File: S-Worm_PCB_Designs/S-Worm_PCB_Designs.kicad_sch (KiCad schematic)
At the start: 25 parts

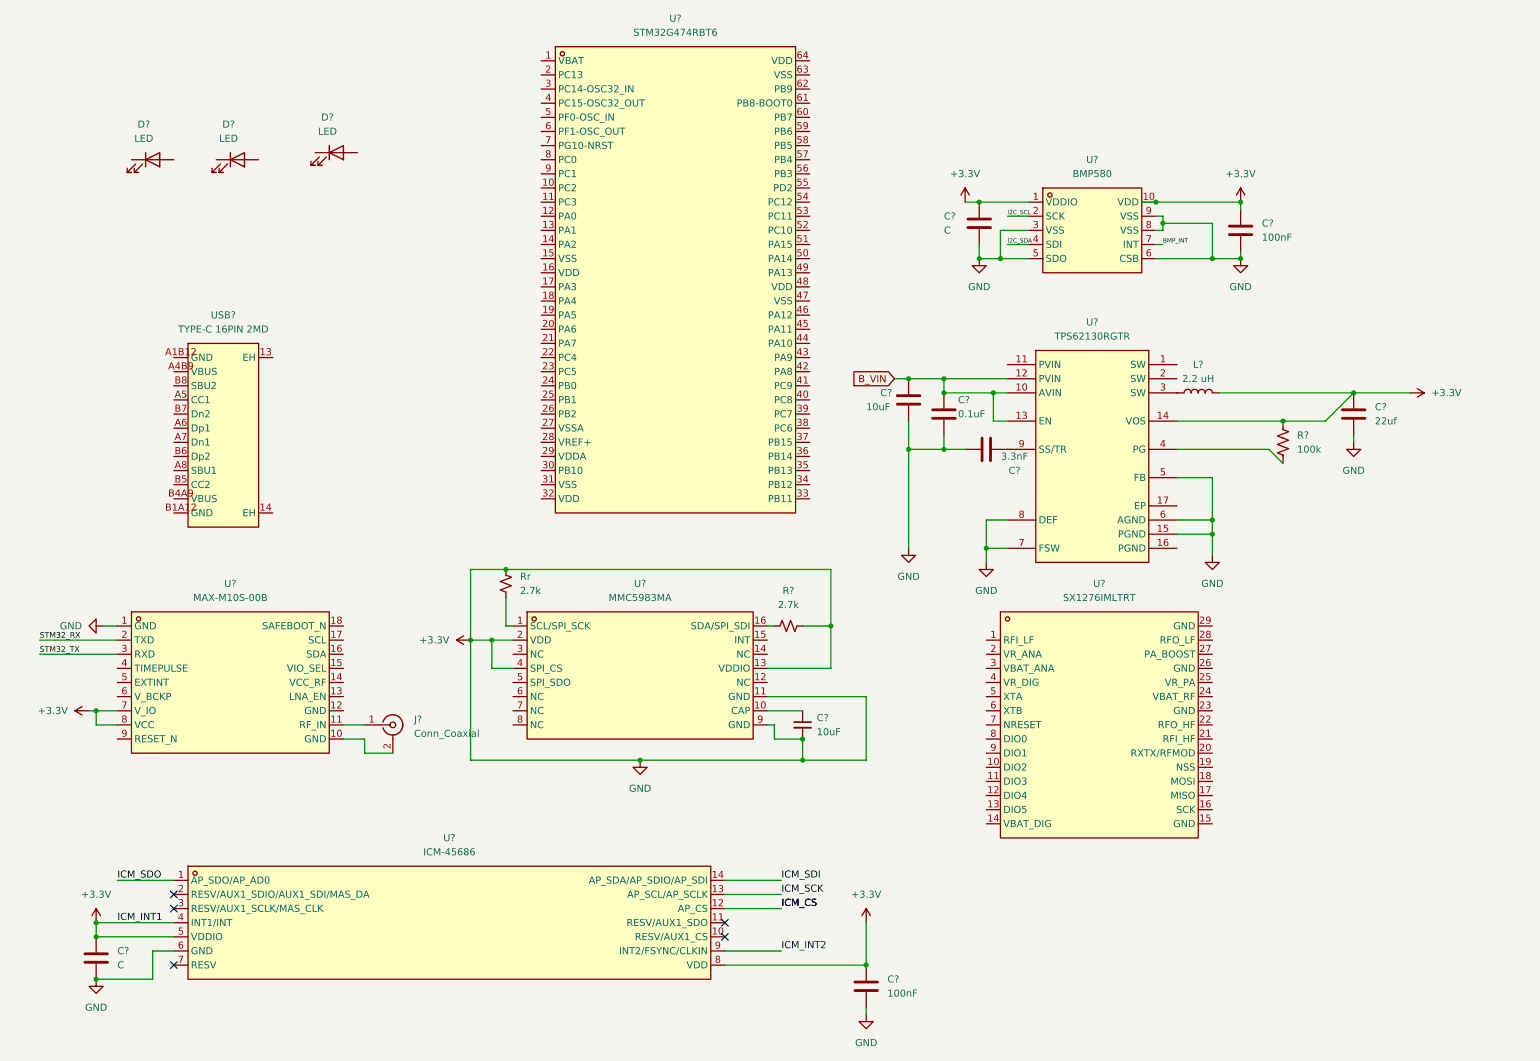
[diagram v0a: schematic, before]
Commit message: power_aaa
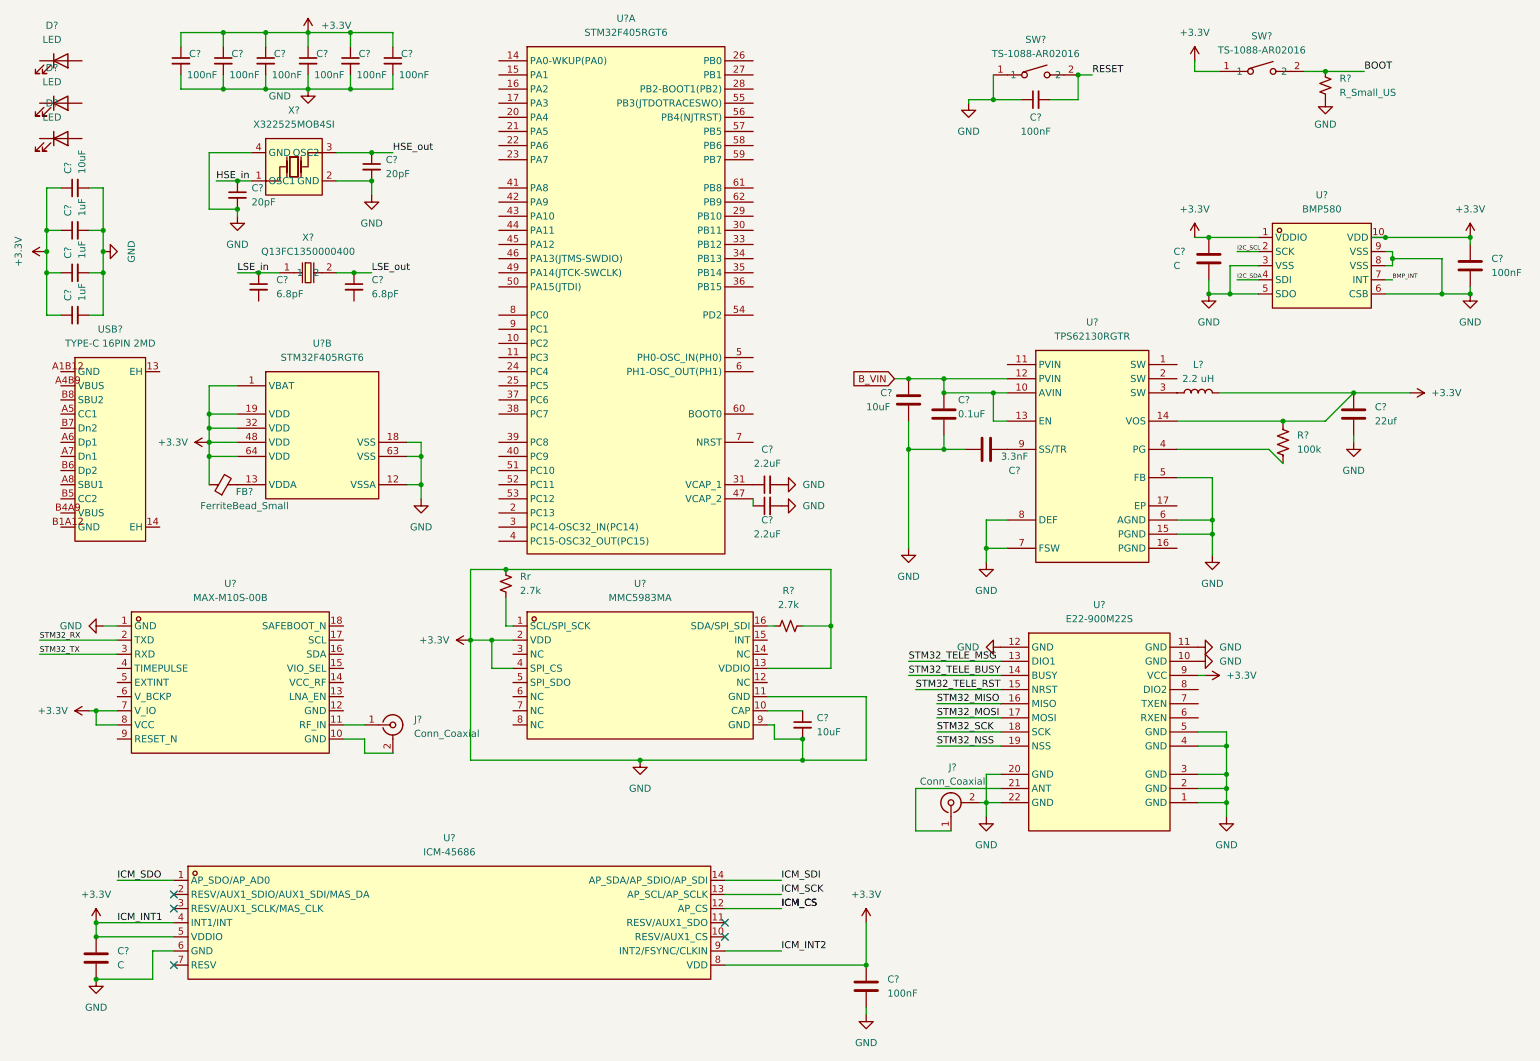
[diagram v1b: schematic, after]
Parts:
- removed U?: SX1276IMLTRT, easyeda2kicad:QFN-28_L6.0-W6.0-P0.65-BL-EP, symbol easyeda2kicad:SX1276IMLTRT
- removed U?: STM32G474RBT6, easyeda2kicad:LQFP-64_L10.0-W10.0-P0.50-LS12.0-BL, symbol easyeda2kicad:STM32G474RBT6
- added C? (x2): 2.2uF, symbol Device:C_Small
- added C?: 10uF, symbol Device:C_Small
- added C? (x7): 100nF, symbol Device:C_Small
- added C? (x3): 1uF, symbol Device:C_Small
- added C? (x2): 6.8pF, symbol Device:C_Small
- added C? (x2): 20pF, symbol Device:C_Small
- added FB?: FerriteBead_Small, symbol Device:FerriteBead_Small
- added J?: Conn_Coaxial, symbol Connector:Conn_Coaxial
- added R?: R_Small_US, symbol Device:R_Small_US
- added SW? (x2): TS-1088-AR02016, easyeda2kicad:SW-SMD_L3.9-W3.0-P4.45, symbol easyeda2kicad:TS-1088-AR02016
- added U? (x2): STM32F405RGT6, easyeda2kicad:LQFP-64_L10.0-W10.0-P0.50-LS12.0-BL, symbol easyeda2kicad:STM32F405RGT6
- added U?: E22-900M22S, easyeda2kicad:WIRELM-SMD_E22-900M22S, symbol easyeda2kicad:E22-900M22S
- added X?: X322525MOB4SI, easyeda2kicad:CRYSTAL-SMD_4P-L3.2-W2.5-BL, symbol easyeda2kicad:X322525MOB4SI
- added X?: Q13FC1350000400, easyeda2kicad:FC-135R_L3.2-W1.5, symbol easyeda2kicad:Q13FC1350000400
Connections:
- net +3.3V: now also C?.1, C?.1, C?.1, C?.1, C?.1, C?.1, C?.1, C?.1, C?.1, C?.1, C?.1, C?.2, C?.2, C?.2, C?.2, C?.2, C?.2, C?.2, C?.2, C?.2, C?.2, C?.2, C?.2, C?.2, C?.2, FB?.1, J?.2 (Ext), R?.2, SW?.1, SW?.1, U?.1 (GND), U?.1 (VBAT), U?.10 (GND), U?.11 (GND), U?.12 (GND), U?.12 (VSSA), U?.18 (VSS), U?.19 (VDD), U?.2 (GND), U?.20 (GND), U?.22 (GND), U?.3 (GND), U?.32 (VDD), U?.4 (GND), U?.48 (VDD), U?.5 (GND), U?.63 (VSS), U?.64 (VDD), U?.9 (VCC), X?.2 (GND), X?.4 (GND)
- new net: C?.1, U?.31 (VCAP_1)
- new net: C?.1, U?.47 (VCAP_2)
- new net: FB?.2, U?.13 (VDDA)
- new net: J?.1 (In), U?.21 (ANT)
- new net BOOT: R?.1, SW?.2
- new net HSE_in: C?.1, X?.1 (OSC1)
- new net HSE_out: C?.1, X?.3 (OSC2)
- new net LSE_in: C?.1, X?.1
- new net LSE_out: C?.1, X?.2
- new net RESET: C?.2, SW?.2
- new net STM32_MISO: U?.16 (MISO)
- new net STM32_MOSI: U?.17 (MOSI)
- new net STM32_NSS: U?.19 (NSS)
- new net STM32_SCK: U?.18 (SCK)
- new net STM32_TELE_BUSY: U?.14 (BUSY)
- new net STM32_TELE_MSG: U?.13 (DIO1)
- new net STM32_TELE_RST: U?.15 (NRST)
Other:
- moved on the sheet: C?, D?, U?, USB?

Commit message: erm
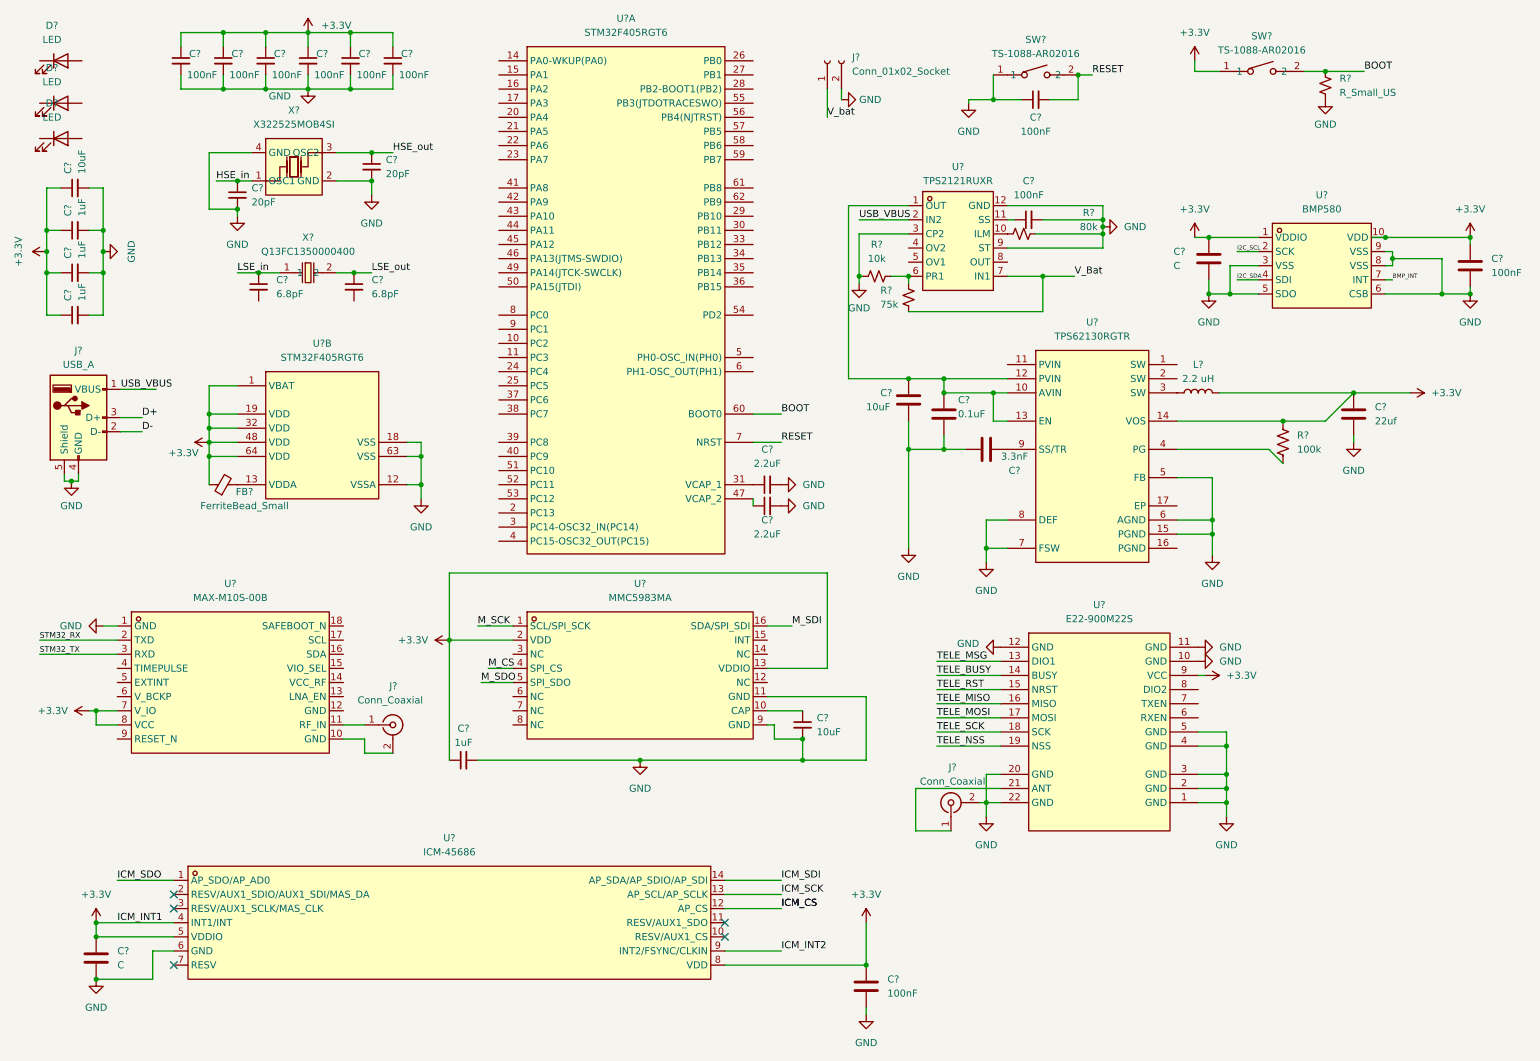
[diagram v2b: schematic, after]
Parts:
- removed R?, Rr: 2.7k, symbol Device:R_Small_US
- removed USB?: TYPE-C 16PIN 2MD, easyeda2kicad:USB-C-SMD_TYPE-C-16PIN-2MD-073, symbol easyeda2kicad:TYPE-C16PIN2MD
- added C?: 1uF, symbol Device:C_Small
- added C?: 100nF, symbol Device:C_Small
- added J?: Conn_01x02_Socket, symbol Connector:Conn_01x02_Socket
- added J?: USB_A, symbol Connector:USB_A
- added R?: 10k, symbol Device:R_Small_US
- added R?: 80k, symbol Device:R_Small_US
- added R?: 75k, symbol Device:R_Small_US
- added U?: TPS2121RUXR, easyeda2kicad:VQFN-HR-12_L2.5-W2.0-P0.50-BL, symbol easyeda2kicad:TPS2121RUXR
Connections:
- net +3.3V: now also C?.1; no longer C?.1, C?.2, C?.2, C?.2, C?.2, C?.2, C?.2, C?.2, C?.2, C?.2, C?.2, C?.2, C?.2, C?.2, C?.2, C?.2, C?.2, C?.2, C?.2, C?.2, C?.2, C?.2, C?.2, C?.2, J?.2 (Ext), R?.2, SW?.1, U?.1 (GND), U?.1 (GND), U?.10 (GND), U?.11 (GND), U?.11 (GND), U?.12 (GND), U?.12 (VSSA), U?.15 (PGND), U?.18 (VSS), U?.2 (GND), U?.20 (GND), U?.22 (GND), U?.3 (GND), U?.3 (VSS), U?.4 (GND), U?.4 (SPI_CS), U?.5 (FB), U?.5 (GND), U?.5 (SDO), U?.6 (AGND), U?.6 (CSB), U?.6 (GND), U?.63 (VSS), U?.7 (FSW), U?.8 (DEF), U?.8 (VSS), U?.9 (GND), U?.9 (VSS), X?.2 (GND), X?.4 (GND)
- net BOOT: now also U?.60 (BOOT0)
- net RESET: now also U?.7 (NRST)
- net M_SDI: now reaches U?.16 (SDA/SPI_SDI)
- net M_SCK: now reaches U?.1 (SCL/SPI_SCK)
- net M_SDO: now reaches U?.5 (SPI_SDO)
- net B_VIN: no longer names the net of C?.1, C?.1, U?.10 (AVIN), U?.12 (PVIN), U?.13 (EN)
- net B_VIN: now also U?.1 (OUT)
- net STM32_MISO renamed TELE_MISO
- net STM32_MOSI renamed TELE_MOSI
- net STM32_NSS renamed TELE_NSS
- net STM32_SCK renamed TELE_SCK
- net STM32_TELE_BUSY renamed TELE_BUSY
- net STM32_TELE_MSG renamed TELE_MSG
- net STM32_TELE_RST renamed TELE_RST
- new net: R?.1, R?.2, U?.6 (PR1)
- new net: R?.1, U?.10 (ILM)
- new net: C?.1, U?.11 (SS)
- new net D+: J?.3 (D+)
- new net D-: J?.2 (D-)
- new net GND: C?.1, C?.2, C?.2, C?.2, C?.2, C?.2, C?.2, C?.2, C?.2, C?.2, C?.2, C?.2, C?.2, C?.2, C?.2, C?.2, C?.2, C?.2, C?.2, C?.2, C?.2, C?.2, C?.2, C?.2, C?.2, C?.2, J?.2 (Ext), J?.2 (Pin_2), J?.4 (GND), J?.5 (Shield), R?.1, R?.2, R?.2, SW?.1, U?.1 (GND), U?.1 (GND), U?.10 (GND), U?.11 (GND), U?.11 (GND), U?.12 (GND), U?.12 (GND), U?.12 (VSSA), U?.15 (PGND), U?.18 (VSS), U?.2 (GND), U?.20 (GND), U?.22 (GND), U?.3 (CP2), U?.3 (GND), U?.3 (VSS), U?.4 (GND), U?.5 (FB), U?.5 (GND), U?.5 (SDO), U?.6 (AGND), U?.6 (CSB), U?.6 (GND), U?.63 (VSS), U?.7 (FSW), U?.8 (DEF), U?.8 (VSS), U?.9 (GND), U?.9 (ST), U?.9 (VSS), X?.2 (GND), X?.4 (GND)
- new net M_CS: U?.4 (SPI_CS)
- new net USB_VBUS: J?.1 (VBUS), U?.2 (IN2)
- new net V_Bat: R?.2, U?.7 (IN1)
- new net V_bat: J?.1 (Pin_1)
